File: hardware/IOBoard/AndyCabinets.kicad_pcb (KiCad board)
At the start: 2 copper layers, 44.4 x 71.4 mm, 52 parts, among them J1 wESP Connector, SW1 Color_Encoder, SW2 Mode_Encoder, U1 74HC14

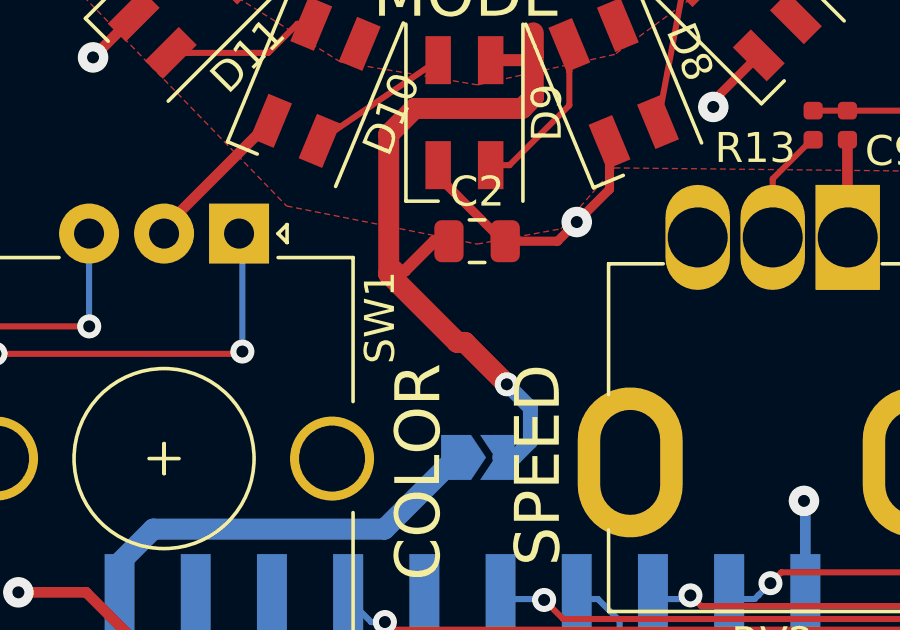
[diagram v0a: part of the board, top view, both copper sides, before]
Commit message: Hardware pre change to SMD2020
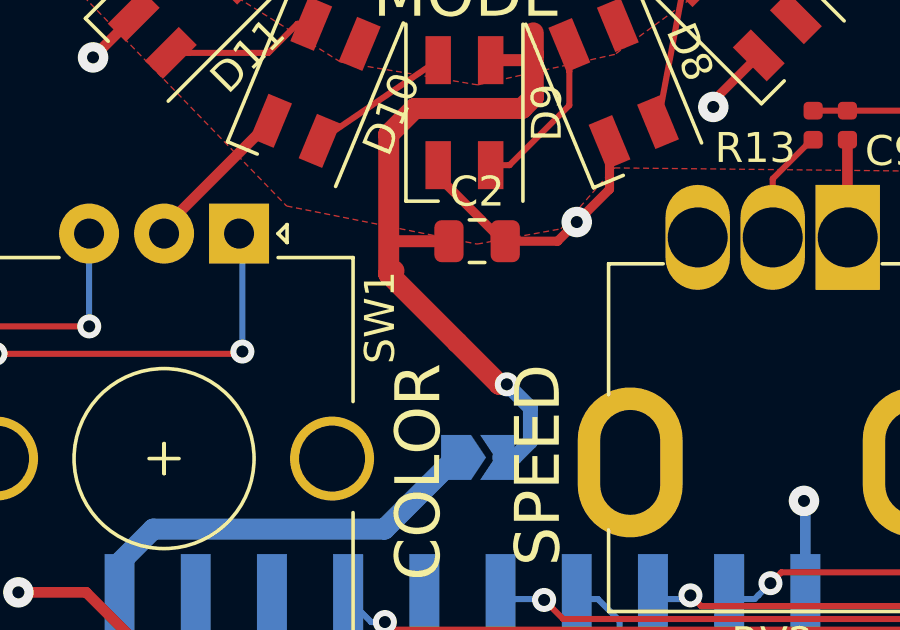
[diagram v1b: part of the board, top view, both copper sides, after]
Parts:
- SW2: footprint Rotary_Encoder:RotaryEncoder_Alps_EC12E-Switch_Vertical_H20mm_CircularMountingHoles -> YonaFootprints:RotaryEncoder_Alps_EC12E-Switch_Vertical_H20mm_CircularMountingHoles_ReducedFootprint
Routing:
- net +5V: track 39.5 -> 40.4 mm
